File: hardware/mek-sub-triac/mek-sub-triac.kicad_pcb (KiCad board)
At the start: 2 copper layers, 25 x 45 mm, 21 parts, among them J1 Conn_01x04_Pin, J2 Screw_Terminal_01x02, Q1 MMBT3904, Q2 BT136S-800E, U1 MOC3063S

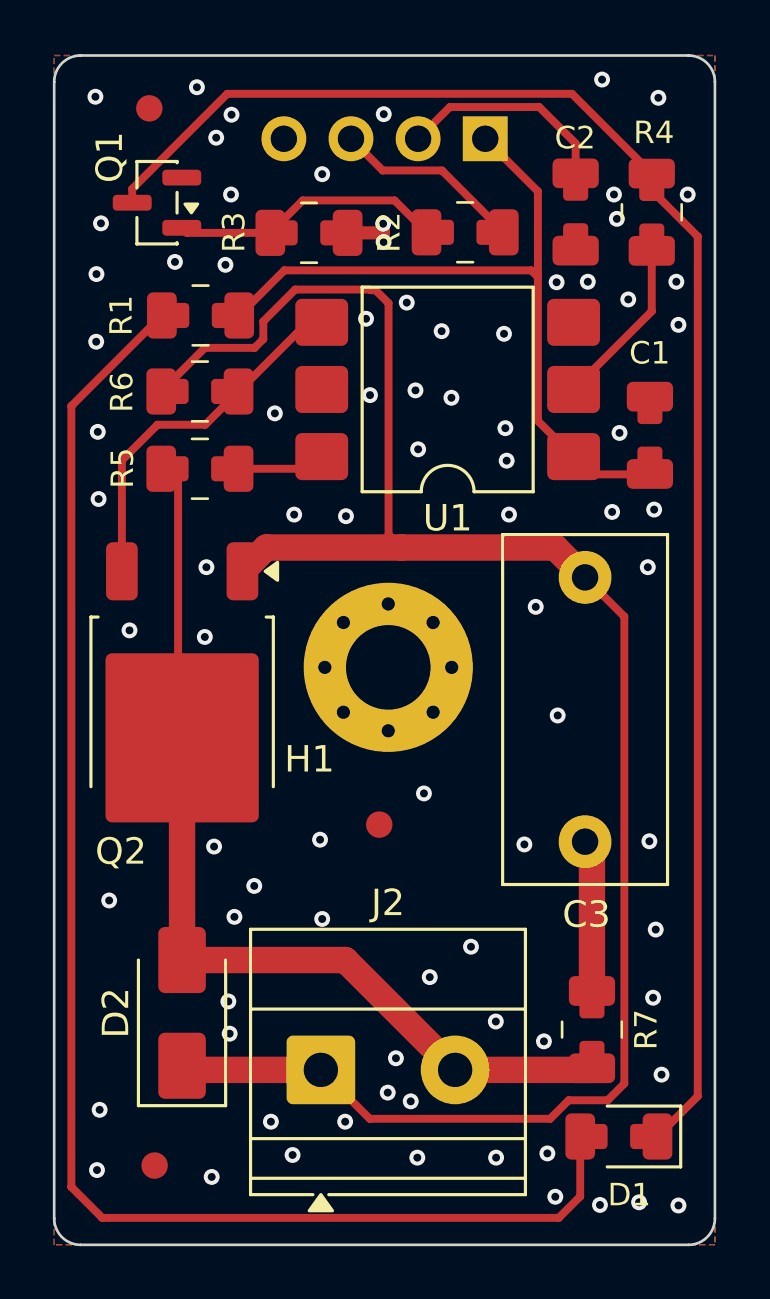
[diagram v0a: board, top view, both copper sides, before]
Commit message: Initial PCB layout
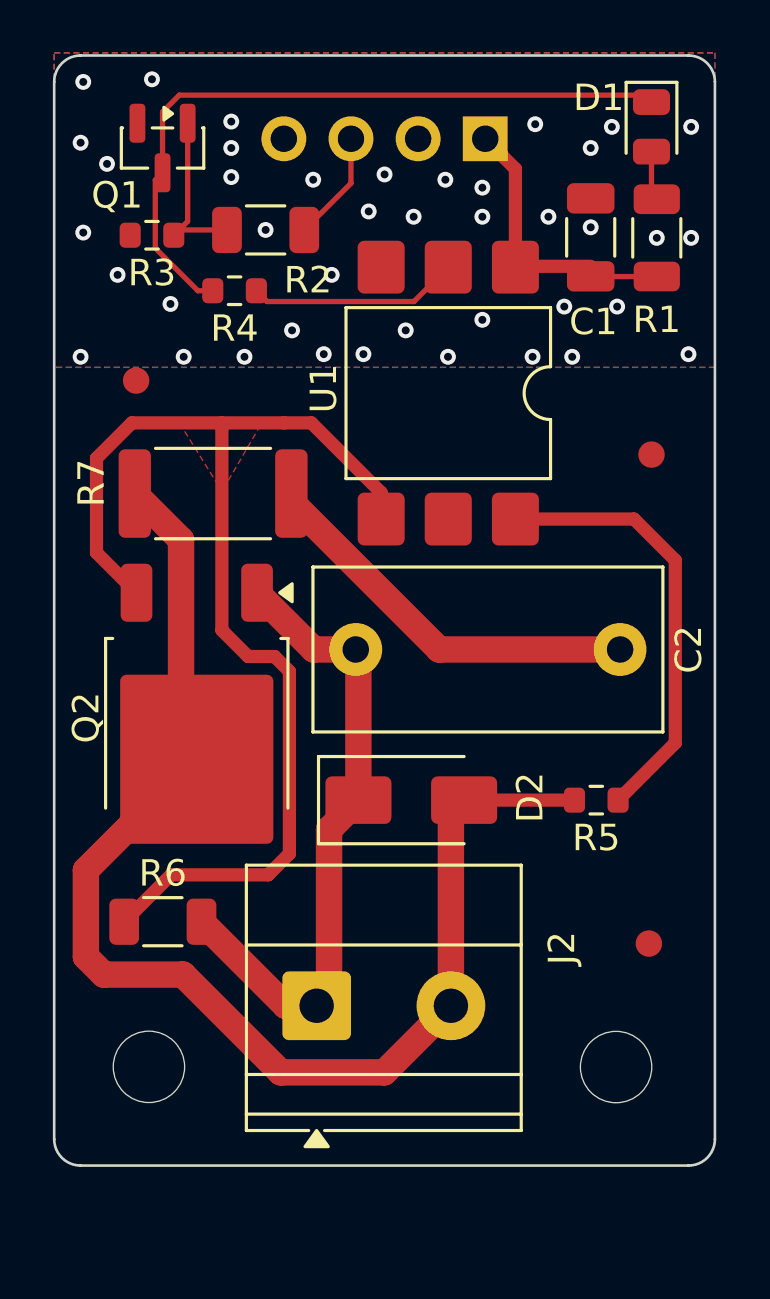
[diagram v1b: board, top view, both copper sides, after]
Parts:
- removed the C2 at (155.7, 85.9)
- added H2: MountingHole_Pad, MountingHole:MountingHole_2.7mm, F.Cu at (157.3, 118.3)
- C1: footprint Mekatrol:C_0603_1206_Combo_Paste0603 -> Capacitor_SMD:C_1206_3216Metric
- D1: footprint Mekatrol:D_0603_1206_Combo_Diode_Paste0603 -> LED_SMD:LED_0805_2012Metric
- H1: footprint MountingHole:MountingHole_3.2mm_M3_Pad_Via -> MountingHole:MountingHole_2.7mm
- R1, R2, R6: footprint Mekatrol:R_0603_1206_Combo_Paste0603 -> Resistor_SMD:R_1206_3216Metric
- R3, R4, R5: footprint Mekatrol:R_0603_1206_Combo_Paste0603 -> Resistor_SMD:R_0603_1608Metric
- R7: footprint Mekatrol:R_0603_1206_Combo_Paste0603 -> Resistor_SMD:R_2512_6332Metric
- moved D1 38.2 mm to (158.6, 82.7), turned to -90 degrees
- moved R7 24.8 mm to (142.0, 96.6), turned to 180 degrees
- moved FID3 20.5 mm to (158.5, 113.6)
- moved R6 20.1 mm to (140.1, 112.8), turned to 0 degrees
- moved R5 19.5 mm to (156.5, 108.2)
- moved H1 17.6 mm to (139.6, 118.3)
- moved R1 17.5 mm to (158.8, 86.9), turned to -90 degrees
- moved FID2 17.4 mm to (158.6, 95.1)
- moved R4 16.1 mm to (142.8, 88.9), turned to 180 degrees
- moved D2 11.8 mm to (149.5, 108.2), turned to 0 degrees
- moved FID1 10.3 mm to (139.1, 92.3)
- moved C1 7.82 mm to (156.3, 86.9)
- moved R2 7.55 mm to (144.0, 86.6)
- moved C2 7.39 mm to (157.4, 102.5), turned to 180 degrees
- moved R3 5.94 mm to (139.7, 86.8), turned to 180 degrees
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- renumbered C3 to C2
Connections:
- net Net-(D2-A1) renamed /MT1
- net Net-(D2-A2) renamed /MT2
- net Net-(Q2-G) renamed /MT1_FB
- net Net-(R5-Pad1) renamed /MT2_FB
- J1 pad 2: +3V3 -> unconnected-(J1-Pin_2-Pad2)
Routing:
- net Net-(D1-A): track 56.7 -> 1.88 mm
- net /MT1: track 71.9 -> 24.5 mm
- net Net-(D1-K): track 60.1 -> 27.0 mm
- net /MT1_FB: track 13.9 -> 44.4 mm
- net +5V: track 28.9 -> 10.9 mm
- net /MT2_FB: track 3.34 -> 16.7 mm
- net /MT2: track 35.9 -> 49.1 mm
- net Net-(C2-Pad1): track 5.76 -> 15.1 mm
- net +3V3: track 8.16 -> 0.00 mm
- net Net-(Q1-B): track 10.3 -> 6.55 mm
- net SIGNAL: track 7.25 -> 4.18 mm
- net GND: track 2.05 -> 0.00 mm, vias 83 -> 41
- net Net-(R4-Pad1): track 6.47 -> 7.97 mm
- added copper zone on F.Cu, net /MT1_FB
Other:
- board size 25 x 45 mm -> 25 x 42 mm
